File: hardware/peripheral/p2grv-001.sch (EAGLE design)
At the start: 5 parts

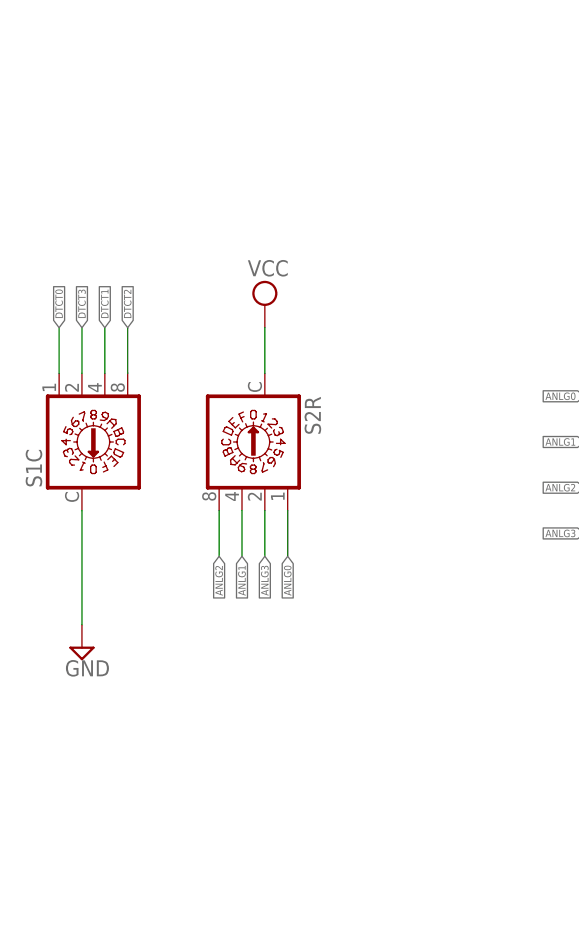
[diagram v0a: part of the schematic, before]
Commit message: WIP.
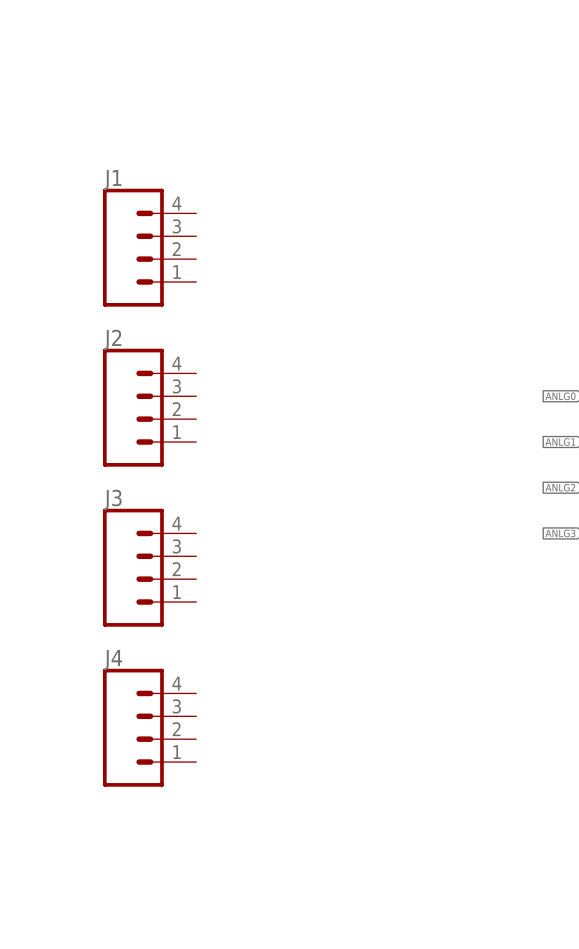
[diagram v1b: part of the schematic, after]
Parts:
- removed S1C, S2R: (no value), switch-dil:A1353HEX
- added J1, J2, J3, J4: (no value), SparkFun-Connectors:CONN_04JST-PTH-VERT
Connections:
- net ANLG0: no longer S2R.1
- net ANLG1: no longer S2R.4
- net ANLG2: no longer S2R.8
- net ANLG3: no longer S2R.2
- net DTCT0: no longer S1C.1
- net DTCT1: no longer S1C.4
- net DTCT2: no longer S1C.8
- net DTCT3: no longer S1C.2
- net GND: no longer S1C.C
- net VCC: no longer S2R.C
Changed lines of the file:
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@@
 <part name="LOGO1" library="SparkFun-Aesthetics" deviceset="OSHW-LOGO" device="S-COPPER" value="OSHW-LOGOS-COPPER"/>
 <part name="JP1" library="pinhead" library_urn="urn:adsk.eagle:library:325" deviceset="PINHD-2X8" device="" package3d_urn="urn:adsk.eagle:package:22481/2"/>
-<part name="S1C" library="switch-dil" library_urn="urn:adsk.eagle:library:375" deviceset="A1353HEX" device="" package3d_urn="urn:adsk.eagle:package:27207/1"/>
-<part name="S2R" library="switch-dil" library_urn="urn:adsk.eagle:library:375" deviceset="A1353HEX" device="" package3d_urn="urn:adsk.eagle:package:27207/1"/>
 <part name="SUPPLY1" library="supply2" library_urn="urn:adsk.eagle:library:372" deviceset="GND" device=""/>
-<part name="SUPPLY2" library="supply2" library_urn="urn:adsk.eagle:library:372" deviceset="GND" device=""/>
 <part name="SUPPLY3" library="supply2" library_urn="urn:adsk.eagle:library:372" deviceset="VCC" device=""/>
-<part name="SUPPLY4" library="supply2" library_urn="urn:adsk.eagle:library:372" deviceset="VCC" device=""/>
 <part name="U$1" library="pineapple" deviceset="PINEAPPLE450_SILK" device=""/>
+<part name="J1" library="SparkFun-Connectors" library_urn="urn:adsk.eagle:library:513" deviceset="CONN_04" device="JST-PTH-VERT" package3d_urn="urn:adsk.eagle:package:38102/1"/>
+<part name="J2" library="SparkFun-Connectors" library_urn="urn:adsk.eagle:library:513" deviceset="CONN_04" device="JST-PTH-VERT" package3d_urn="urn:adsk.eagle:package:38102/1"/>
+<part name="J3" library="SparkFun-Connectors" library_urn="urn:adsk.eagle:library:513" deviceset="CONN_04" device="JST-PTH-VERT" package3d_urn="urn:adsk.eagle:package:38102/1"/>
+<part name="J4" library="SparkFun-Connectors" library_urn="urn:adsk.eagle:library:513" deviceset="CONN_04" device="JST-PTH-VERT" package3d_urn="urn:adsk.eagle:package:38102/1"/>
 </parts>
 <sheets>
@@
 <attribute name="VALUE" x="105.41" y="86.36" size="1.778" layer="96"/>
 </instance>
-<instance part="S1C" gate="1" x="40.64" y="101.6" smashed="yes">
-<attribute name="NAME" x="36.195" y="96.52" size="1.778" layer="95" rot="R90"/>
-<attribute name="VALUE" x="49.53" y="96.52" size="1.778" layer="96" rot="R90"/>
-</instance>
-<instance part="S2R" gate="1" x="60.96" y="101.6" smashed="yes" rot="R180">
-<attribute name="NAME" x="65.405" y="106.68" size="1.778" layer="95" rot="R270"/>
-<attribute name="VALUE" x="52.07" y="106.68" size="1.778" layer="96" rot="R270"/>
-</instance>
 <instance part="SUPPLY1" gate="GND" x="101.6" y="73.66" smashed="yes">
 <attribute name="VALUE" x="99.695" y="70.485" size="1.778" layer="96"/>
-</instance>
-<instance part="SUPPLY2" gate="GND" x="40.64" y="78.74" smashed="yes">
-<attribute name="VALUE" x="38.735" y="75.565" size="1.778" layer="96"/>
 </instance>
 <instance part="SUPPLY3" gate="G$1" x="124.46" y="127" smashed="yes">
 <attribute name="VALUE" x="122.555" y="130.175" size="1.778" layer="96"/>
 </instance>
-<instance part="SUPPLY4" gate="G$1" x="60.96" y="116.84" smashed="yes">
-<attribute name="VALUE" x="59.055" y="120.015" size="1.778" layer="96"/>
+<instance part="U$1" gate="G$1" x="241.3" y="142.24" smashed="yes"/>
+<instance part="J1" gate="G$1" x="48.26" y="121.92" smashed="yes">
+<attribute name="VALUE" x="43.18" y="114.554" size="1.778" layer="96" font="vector"/>
+<attribute name="NAME" x="43.18" y="130.048" size="1.778" layer="95" font="vector"/>
 </instance>
-<instance part="U$1" gate="G$1" x="241.3" y="142.24" smashed="yes"/>
+<instance part="J2" gate="G$1" x="48.26" y="104.14" smashed="yes">
+<attribute name="VALUE" x="43.18" y="96.774" size="1.778" layer="96" font="vector"/>
+<attribute name="NAME" x="43.18" y="112.268" size="1.778" layer="95" font="vector"/>
+</instance>
+<instance part="J3" gate="G$1" x="48.26" y="86.36" smashed="yes">
+<attribute name="VALUE" x="43.18" y="78.994" size="1.778" layer="96" font="vector"/>
+<attribute name="NAME" x="43.18" y="94.488" size="1.778" layer="95" font="vector"/>
+</instance>
+<instance part="J4" gate="G$1" x="48.26" y="68.58" smashed="yes">
+<attribute name="VALUE" x="43.18" y="61.214" size="1.778" layer="96" font="vector"/>
+<attribute name="NAME" x="43.18" y="76.708" size="1.778" layer="95" font="vector"/>
+</instance>
 </instances>
 <busses>
@@
 <junction x="101.6" y="93.98"/>
 </segment>
-<segment>
-<pinref part="S1C" gate="1" pin="C"/>
-<wire x1="40.64" y1="93.98" x2="40.64" y2="81.28" width="0.1524" layer="91"/>
-<pinref part="SUPPLY2" gate="GND" pin="GND"/>
-</segment>
 </net>
 <net name="DTCT0" class="0">
@@
 <wire x1="116.84" y1="109.22" x2="132.08" y2="109.22" width="0.1524" layer="91"/>
 <label x="132.08" y="109.22" size="0.8128" layer="95" xref="yes"/>
-</segment>
-<segment>
-<pinref part="S1C" gate="1" pin="1"/>
-<wire x1="38.1" y1="109.22" x2="38.1" y2="114.3" width="0.1524" layer="91"/>
-<label x="38.1" y="114.3" size="0.8128" layer="95" rot="R90" xref="yes"/>
 </segment>
 </net>
@@
 <junction x="124.46" y="101.6"/>
 </segment>
-<segment>
-<pinref part="S2R" gate="1" pin="C"/>
-<wire x1="60.96" y1="109.22" x2="60.96" y2="114.3" width="0.1524" layer="91"/>
-<pinref part="SUPPLY4" gate="G$1" pin="VCC"/>
-</segment>
 </net>
 <net name="DTCT1" class="0">
@@
 <wire x1="116.84" y1="104.14" x2="132.08" y2="104.14" width="0.1524" layer="91"/>
 <label x="132.08" y="104.14" size="0.8128" layer="95" xref="yes"/>
-</segment>
-<segment>
-<pinref part="S1C" gate="1" pin="4"/>
-<wire x1="43.18" y1="109.22" x2="43.18" y2="114.3" width="0.1524" layer="91"/>
-<label x="43.18" y="114.3" size="0.8128" layer="95" rot="R90" xref="yes"/>
 </segment>
 </net>
@@
 <label x="132.08" y="99.06" size="0.8128" layer="95" xref="yes"/>
 </segment>
-<segment>
-<pinref part="S1C" gate="1" pin="8"/>
-<wire x1="45.72" y1="109.22" x2="45.72" y2="114.3" width="0.1524" layer="91"/>
-<label x="45.72" y="114.3" size="0.8128" layer="95" rot="R90" xref="yes"/>
-</segment>
 </net>
 <net name="DTCT3" class="0">
@@
 <wire x1="116.84" y1="93.98" x2="132.08" y2="93.98" width="0.1524" layer="91"/>
 <label x="132.08" y="93.98" size="0.8128" layer="95" xref="yes"/>
-</segment>
-<segment>
-<pinref part="S1C" gate="1" pin="2"/>
-<wire x1="40.64" y1="109.22" x2="40.64" y2="114.3" width="0.1524" layer="91"/>
-<label x="40.64" y="114.3" size="0.8128" layer="95" rot="R90" xref="yes"/>
 </segment>
 </net>
@@
 <label x="96.52" y="106.68" size="0.8128" layer="95" rot="R180" xref="yes"/>
 </segment>
-<segment>
-<pinref part="S2R" gate="1" pin="1"/>
-<wire x1="63.5" y1="93.98" x2="63.5" y2="88.9" width="0.1524" layer="91"/>
-<label x="63.5" y="88.9" size="0.8128" layer="95" rot="R270" xref="yes"/>
-</segment>
 </net>
 <net name="ANLG1" class="0">
@@
 <label x="96.52" y="101.6" size="0.8128" layer="95" rot="R180" xref="yes"/>
 </segment>
-<segment>
-<pinref part="S2R" gate="1" pin="4"/>
-<wire x1="58.42" y1="93.98" x2="58.42" y2="88.9" width="0.1524" layer="91"/>
-<label x="58.42" y="88.9" size="0.8128" layer="95" rot="R270" xref="yes"/>
-</segment>
 </net>
 <net name="ANLG3" class="0">
-<segment>
-<pinref part="S2R" gate="1" pin="2"/>
-<wire x1="60.96" y1="93.98" x2="60.96" y2="88.9" width="0.1524" layer="91"/>
-<label x="60.96" y="88.9" size="0.8128" layer="95" rot="R270" xref="yes"/>
-</segment>
 <segment>
 <pinref part="JP1" gate="A" pin="15"/>
@@
 <net name="ANLG2" class="0">
 <segment>
-<pinref part="S2R" gate="1" pin="8"/>
-<wire x1="55.88" y1="93.98" x2="55.88" y2="88.9" width="0.1524" layer="91"/>
-<label x="55.88" y="88.9" size="0.8128" layer="95" rot="R270" xref="yes"/>
-</segment>
-<segment>
 <pinref part="JP1" gate="A" pin="11"/>
